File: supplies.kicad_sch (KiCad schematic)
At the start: 29 parts, among them J19 KEY_SWITCH, U16 L7805, U17 AMS1117-3.3

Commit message: Update a few library symbols
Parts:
- C78, C83, C85: symbol Device:CP -> Device:C_Polarized
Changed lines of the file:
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@@
     (pin "1")
   )
-  (symbol (lib_id "Device:CP") (at 194.31 46.99 0) (unit 1)
+  (symbol (lib_id "Device:C_Polarized") (at 194.31 46.99 0) (unit 1)
     (in_bom yes) (on_board yes)
     (property "Reference" "C78" (id 0) (at 197.3072 45.8216 0)
@@
     (pin "2")
   )
-  (symbol (lib_id "Device:CP") (at 252.73 44.45 0) (unit 1)
+  (symbol (lib_id "Device:C_Polarized") (at 252.73 44.45 0) (unit 1)
     (in_bom yes) (on_board yes)
     (property "Reference" "C85" (id 0) (at 255.7272 43.2816 0)
@@
     (pin "1")
   )
-  (symbol (lib_id "Device:CP") (at 231.14 95.25 0) (unit 1)
+  (symbol (lib_id "Device:C_Polarized") (at 231.14 95.25 0) (unit 1)
     (in_bom yes) (on_board yes)
     (property "Reference" "C83" (id 0) (at 234.1372 94.0816 0)

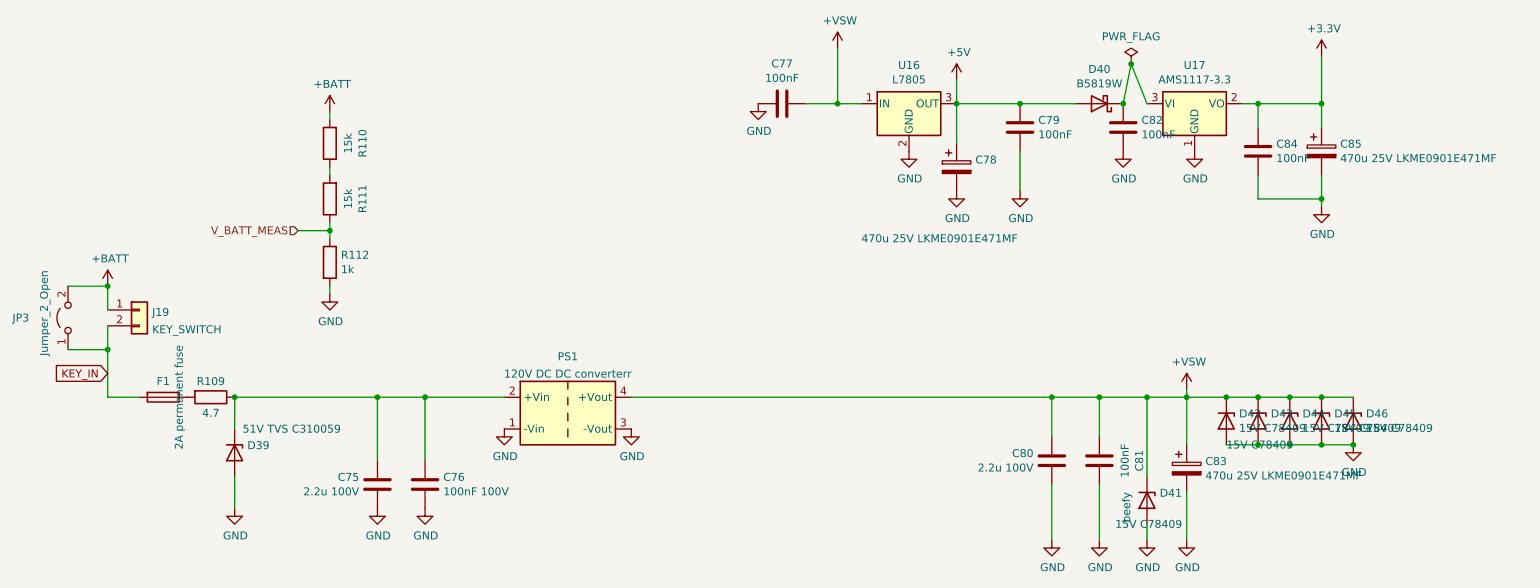
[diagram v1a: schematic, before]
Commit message: Some ERC fixes and other cleanups
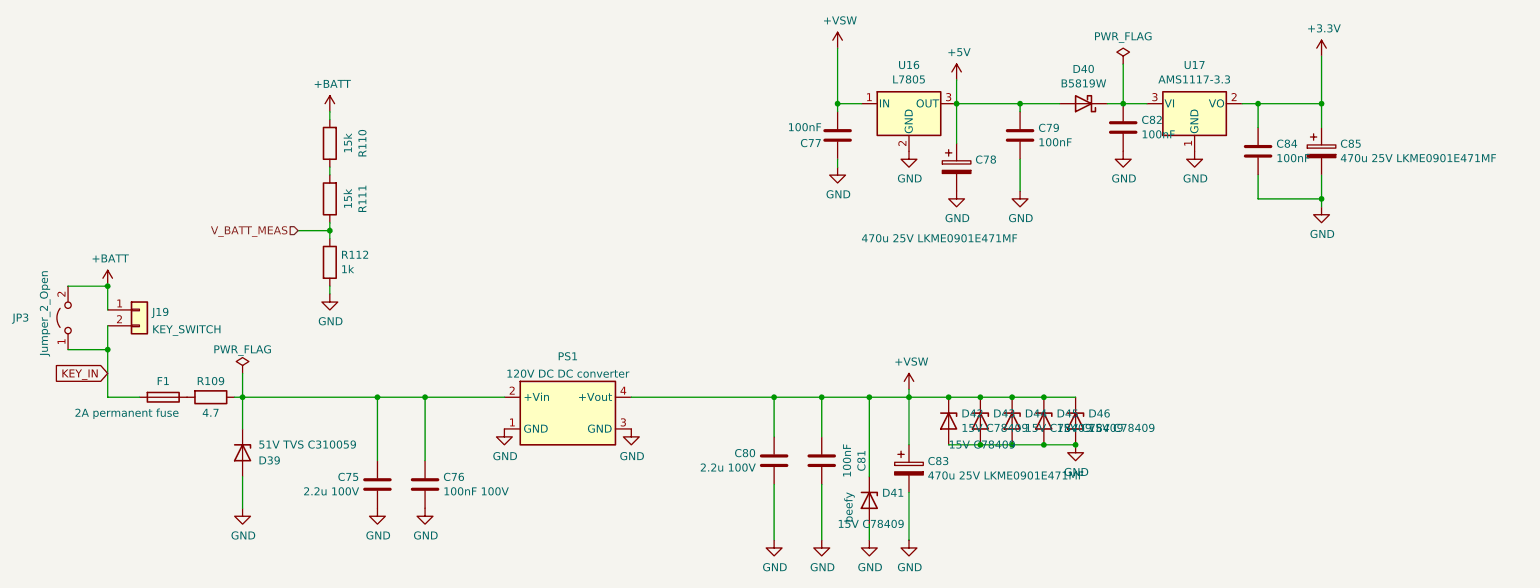
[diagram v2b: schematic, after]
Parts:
- PS1: value 120V DC DC converterr -> 120V DC DC converter; symbol Converter_DCDC:MEE1S0303SC -> Bobbycontroller:120V_DCDC
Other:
- moved on the sheet: C77, C79, C80, C81, C83, D39, D40, D41, D42, D43, D44, D45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
